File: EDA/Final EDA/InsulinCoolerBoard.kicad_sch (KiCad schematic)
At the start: 0 parts

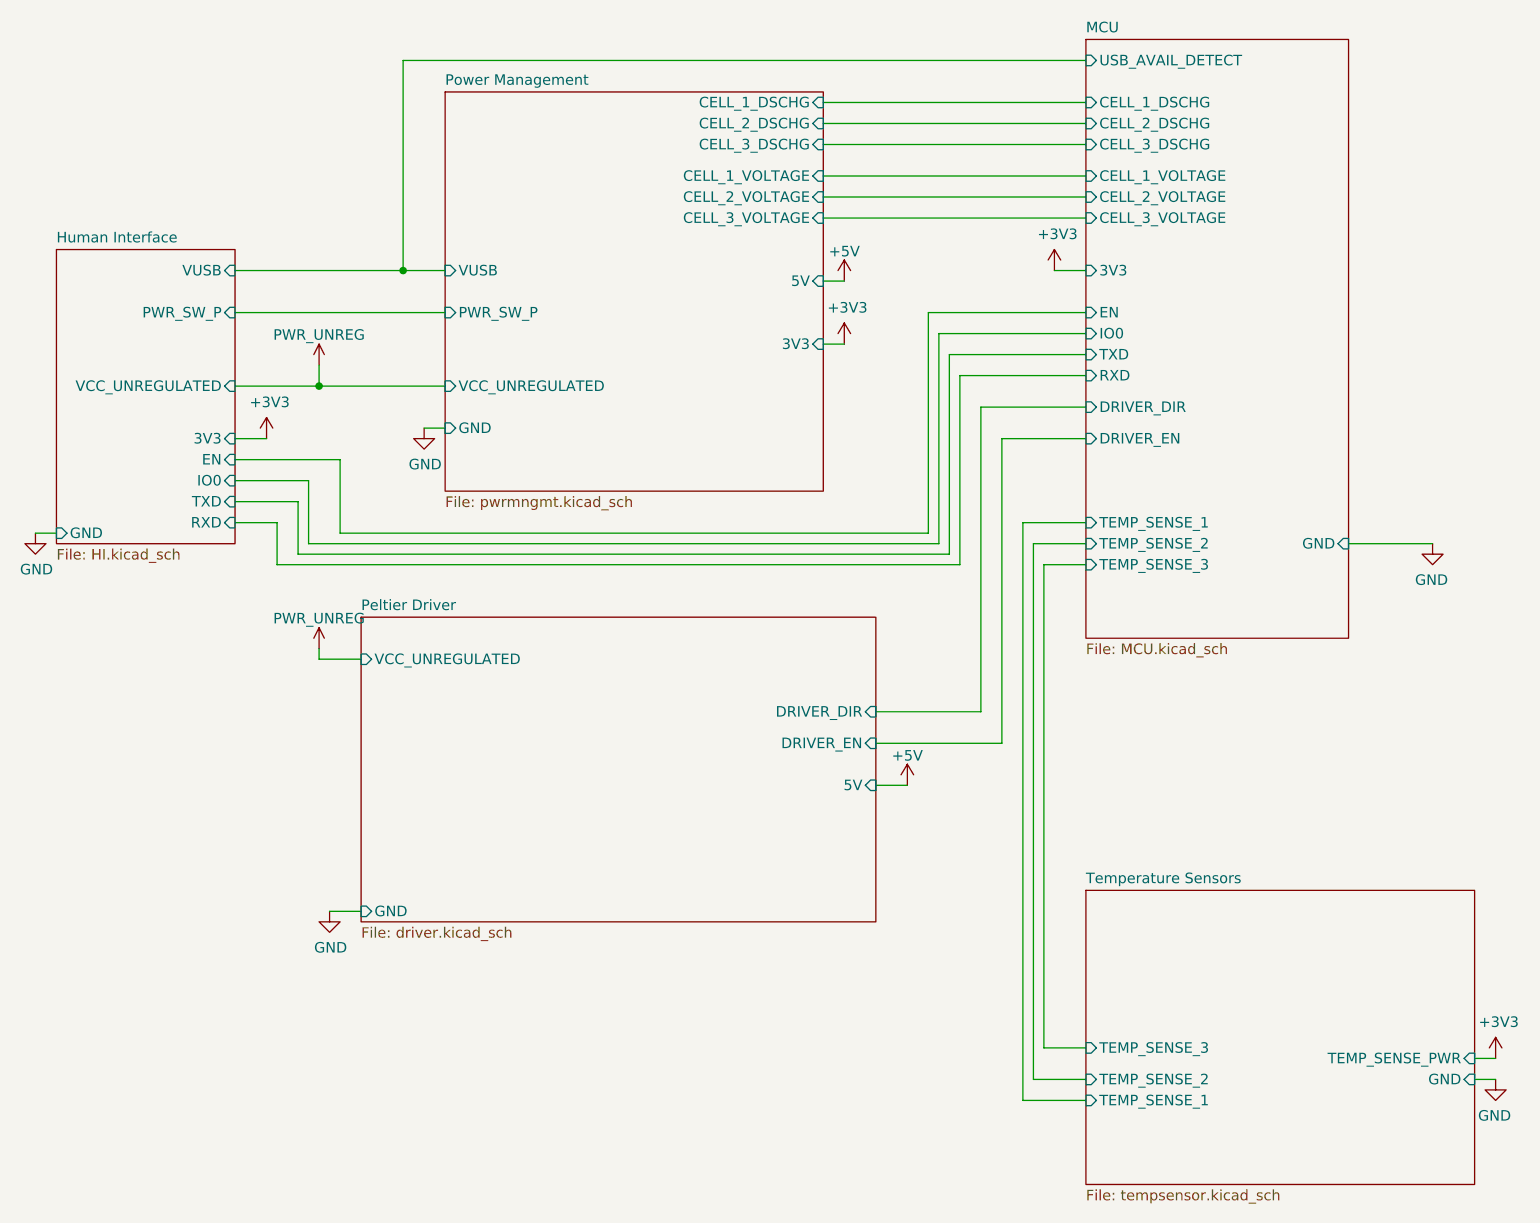
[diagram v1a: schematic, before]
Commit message: e
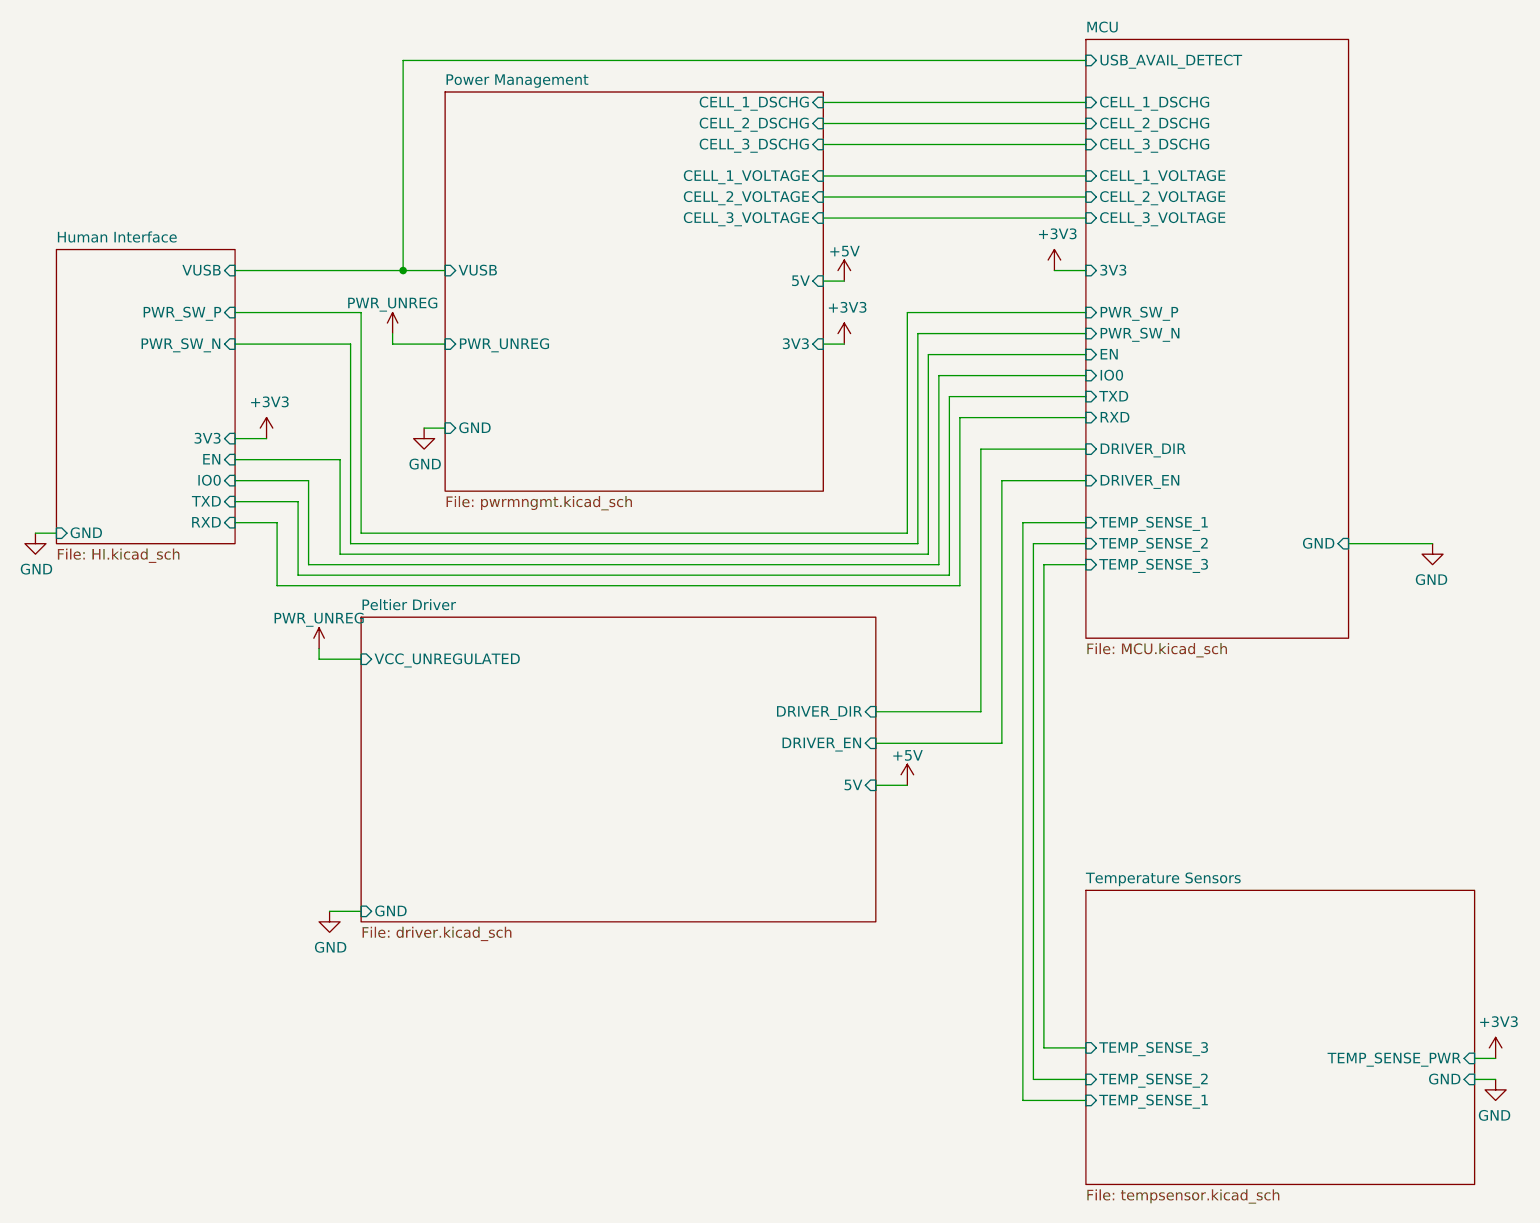
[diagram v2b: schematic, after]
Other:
- sheet Human Interface ports: added PWR_SW_N; removed VCC_UNREGULATED
- sheet MCU ports: added PWR_SW_N, PWR_SW_P; removed none
- sheet Power Management ports: added PWR_UNREG; removed PWR_SW_P, VCC_UNREGULATED
